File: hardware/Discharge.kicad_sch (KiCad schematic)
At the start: 5 parts, among them Q4 CPH3351

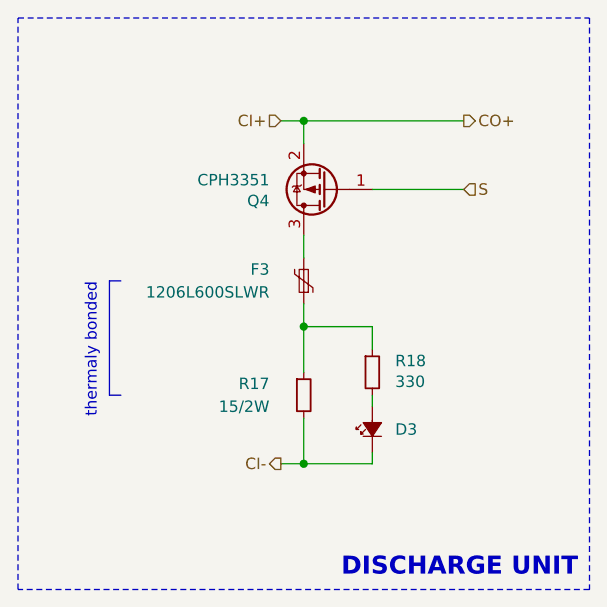
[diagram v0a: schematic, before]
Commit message: new schematic
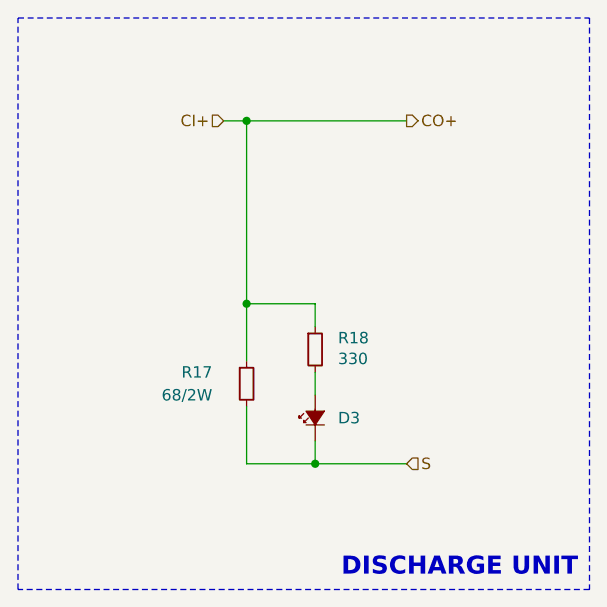
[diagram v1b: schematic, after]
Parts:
- removed F3: 1206L600SLWR, Fuse:Fuse_2512_6332Metric, symbol 1206l600slwr:1206L600SLWR
- removed Q4: CPH3351, Package_TO_SOT_SMD:SOT-23, symbol PUTM_EV_BMS_HV_Slave_2021-rescue:Q_PMOS_GSD-Device
- R17: value 15/2W -> 68/2W; CBOM HP2512-15R -> (none); Manufacturer_Part_Number CRM2512QFW-10R0ELF -> CR2512-JW-680ELF; Mouser Part Number 652-CRM2512QFW-10R0E -> 652-CR2512-JW-680ELF; Mouser Price/Stock https://www.mouser.pl/ProductDetail/Bourns/CRM2512QFW-10R0E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 -> https://www.mouser.pl/ProductDetail/Bourns/CR2512-JW-680ELF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
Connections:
- net CI- is gone; now on net S: D3.1 (K), R17.2
- net CI+: now also R17.1, R18.1
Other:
- note removed: "thermaly bonded"
- moved on the sheet: D3, R17, R18
